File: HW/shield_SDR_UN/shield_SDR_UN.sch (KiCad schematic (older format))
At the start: 0 parts

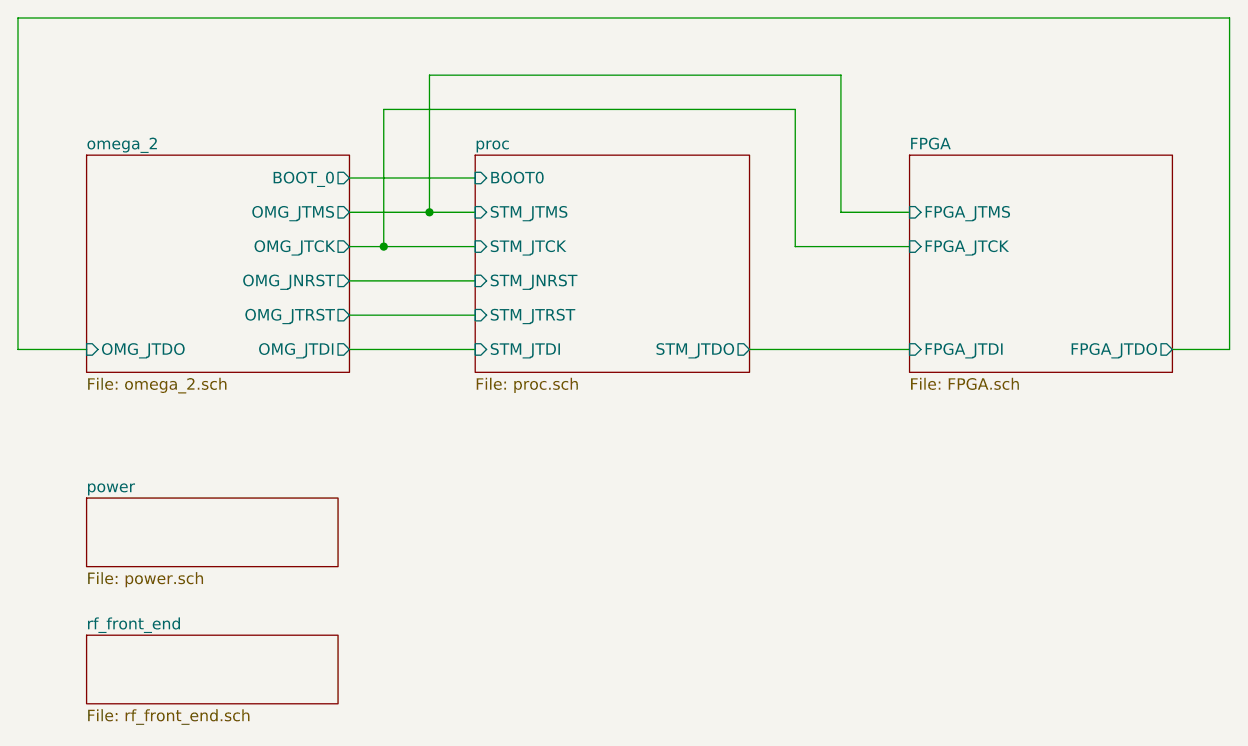
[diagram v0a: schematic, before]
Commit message: i2c_complete
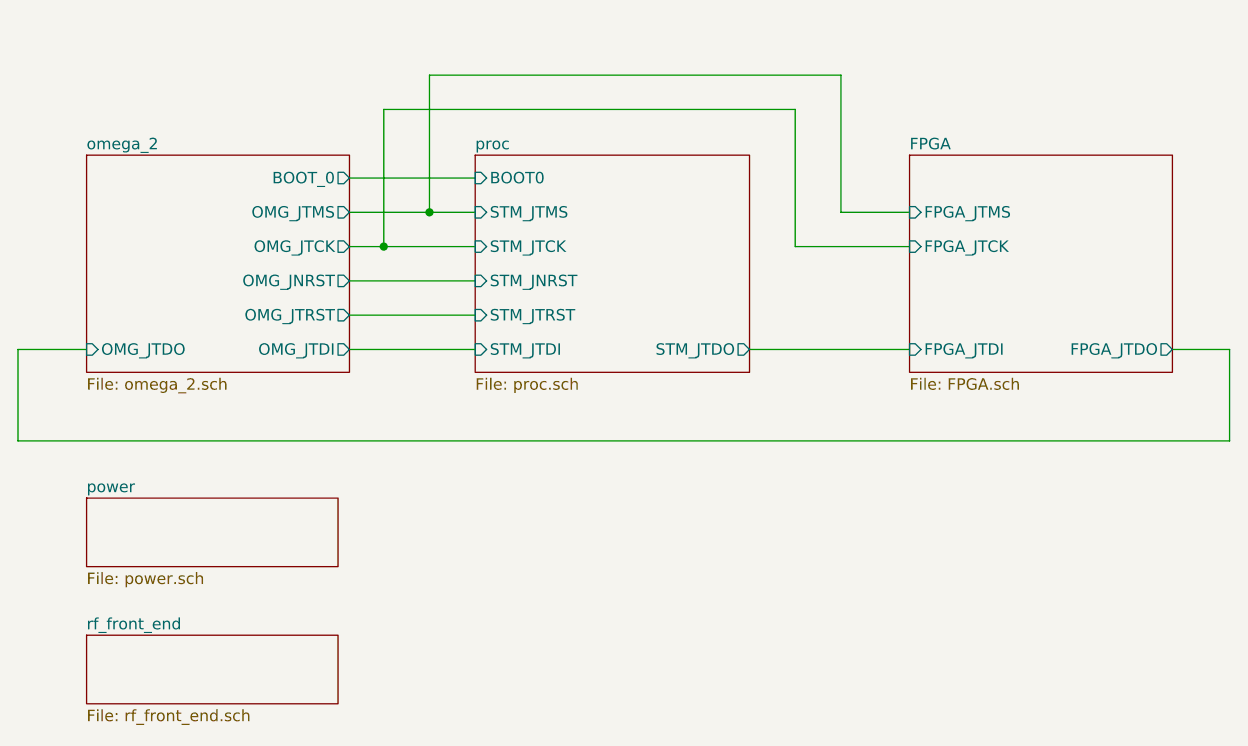
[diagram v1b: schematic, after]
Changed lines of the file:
@@
 	9000 3850 9250 3850
 Wire Wire Line
-	9250 3850 9250 2400
+	3950 3850 4250 3850
 Wire Wire Line
-	9250 2400 3950 2400
+	3950 3850 3950 4250
 Wire Wire Line
-	3950 2400 3950 3850
+	3950 4250 9250 4250
 Wire Wire Line
-	3950 3850 4250 3850
+	9250 4250 9250 3850
 $EndSCHEMATC
